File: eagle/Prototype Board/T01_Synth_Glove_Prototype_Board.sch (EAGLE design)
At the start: 61 parts, among them SW1 RESET_BUTTON, U1 ATMEGA328P, U2 ZLDO1117

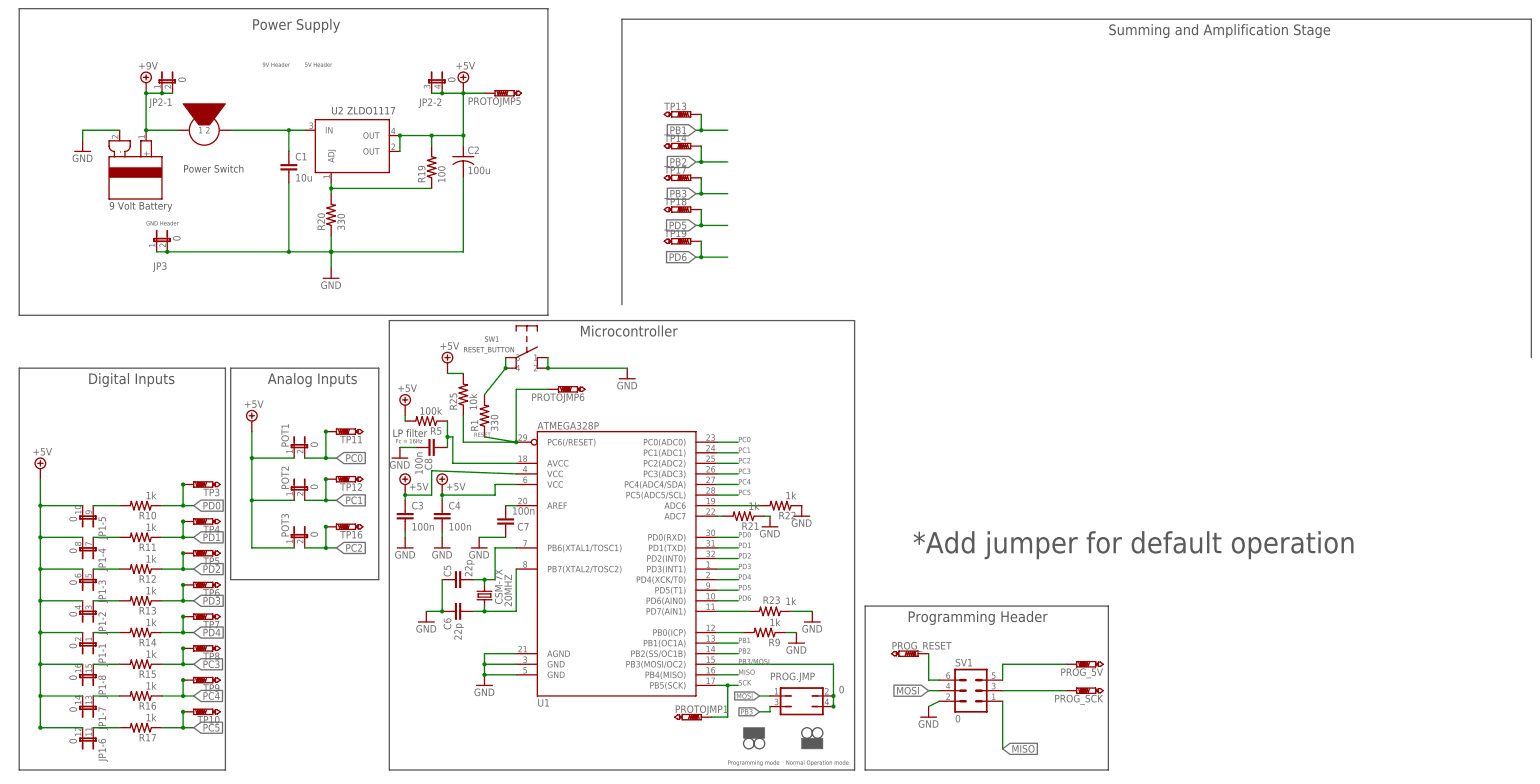
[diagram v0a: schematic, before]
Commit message: Revisions and more CAM
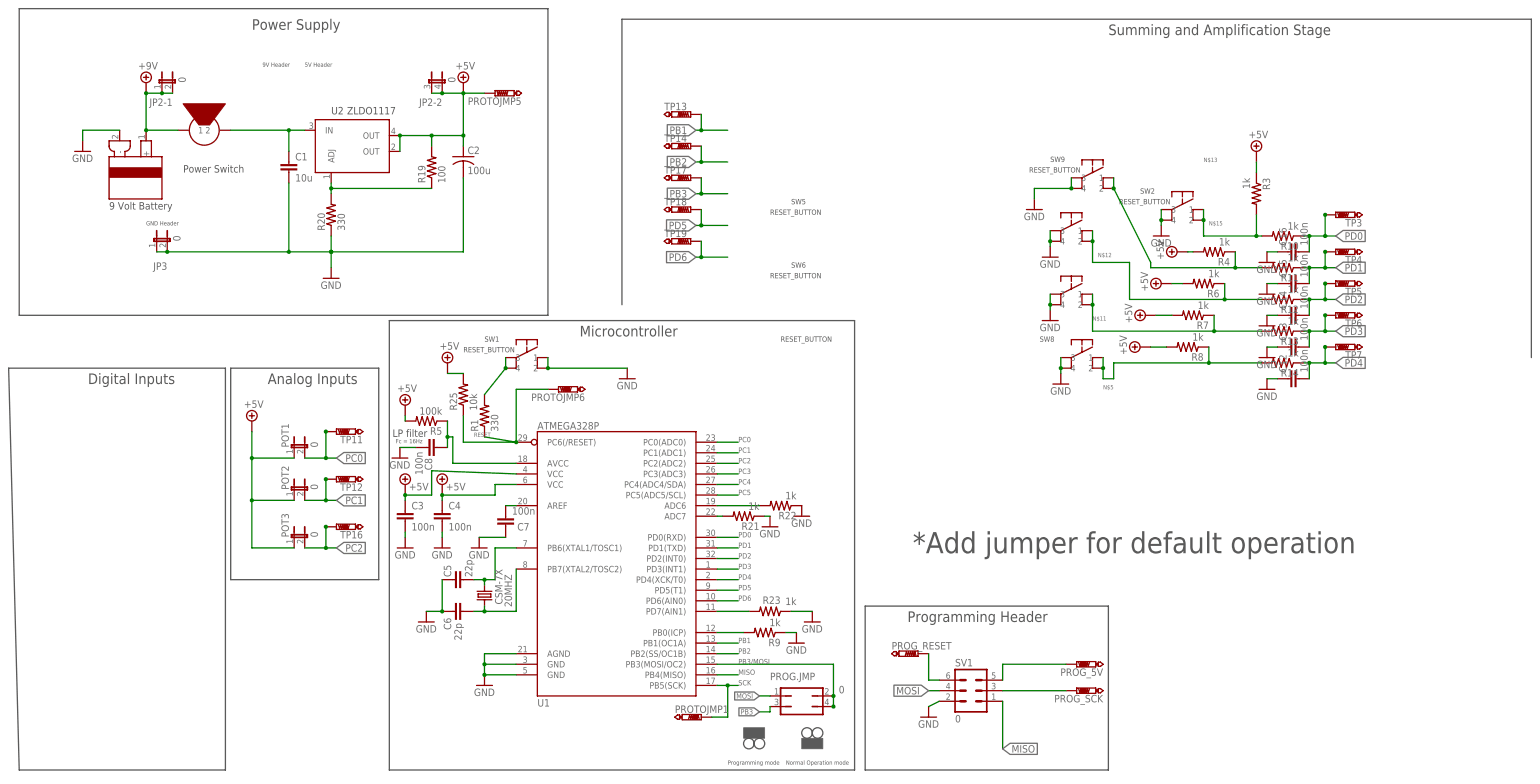
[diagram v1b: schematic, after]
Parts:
- removed JP1: 0, jumper:JP8QE
- removed R15, R16, R17: 1k, SparkFun-Resistors:RESISTOR0603
- removed TP10, TP8, TP9: PTR1B2,54, testpad:PTR1B2,54
- added C12, C13, C14, C15, C16: 100n, SparkFun-Capacitors:CAP0603-CAP
- added R3, R4, R6, R7, R8: 1k, SparkFun-Resistors:RESISTOR0603
- added SW2, SW5, SW6, SW8, SW9: RESET_BUTTON, Synth_Glove:RESET_BUTTON
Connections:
- removed net N$23: JP1-6.1, R17.2
- removed net N$3: JP1-5.1, R10.2
- removed net N$4: JP1-4.1, R11.2
- net +5V: now also R3.1, R4.2, R6.2, R7.2, R8.2; no longer JP1-1.2, JP1-2.2, JP1-3.2, JP1-4.2, JP1-5.2, JP1-6.2, JP1-7.2, JP1-8.2
- net GND: now also C12.1, C13.1, C14.1, C15.1, C16.1, SW2.3, SW2.4, SW5.3, SW5.4, SW6.3, SW6.4, SW8.3, SW8.4, SW9.3, SW9.4
- net N$11: now also R7.1, SW6.1, SW6.2; no longer JP1-2.1
- net N$12: now also R12.2, R6.1, SW5.1, SW5.2; no longer JP1-1.1, R14.2
- net N$13: now also R11.2, R4.1, SW9.1, SW9.2; no longer JP1-8.1, R15.2
- net N$15: now also R10.2, R3.2, SW2.1, SW2.2; no longer JP1-7.1, R16.2
- net N$5: now also R14.2, R8.1, SW8.1, SW8.2; no longer JP1-3.1, R12.2
- net PC3: no longer R15.1, TP8.TP
- net PC4: no longer R16.1, TP9.TP
- net PC5: no longer R17.1, TP10.TP
- net PD0: now also C16.2
- net PD1: now also C15.2
- net PD2: now also C14.2
- net PD3: now also C13.2
- net PD4: now also C12.2
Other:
- moved on the sheet: R10, R11, R12, R13, R14, TP3, TP4, TP5, TP6, TP7
